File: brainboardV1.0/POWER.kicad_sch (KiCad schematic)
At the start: 16 parts, among them J21 Conn_01x01, J22 Conn_01x01, J23 Conn_01x01, U21 LD1117S18TR_SOT223

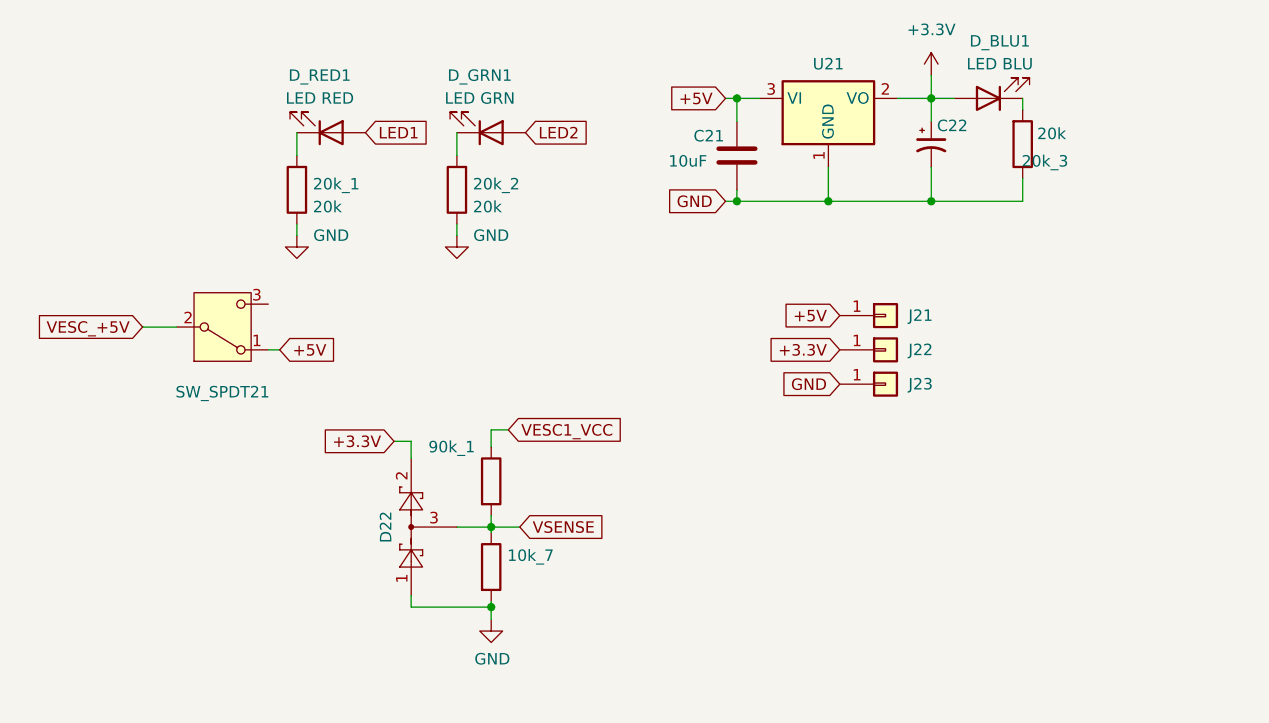
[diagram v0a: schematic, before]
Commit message: finalized PCB, changed file names
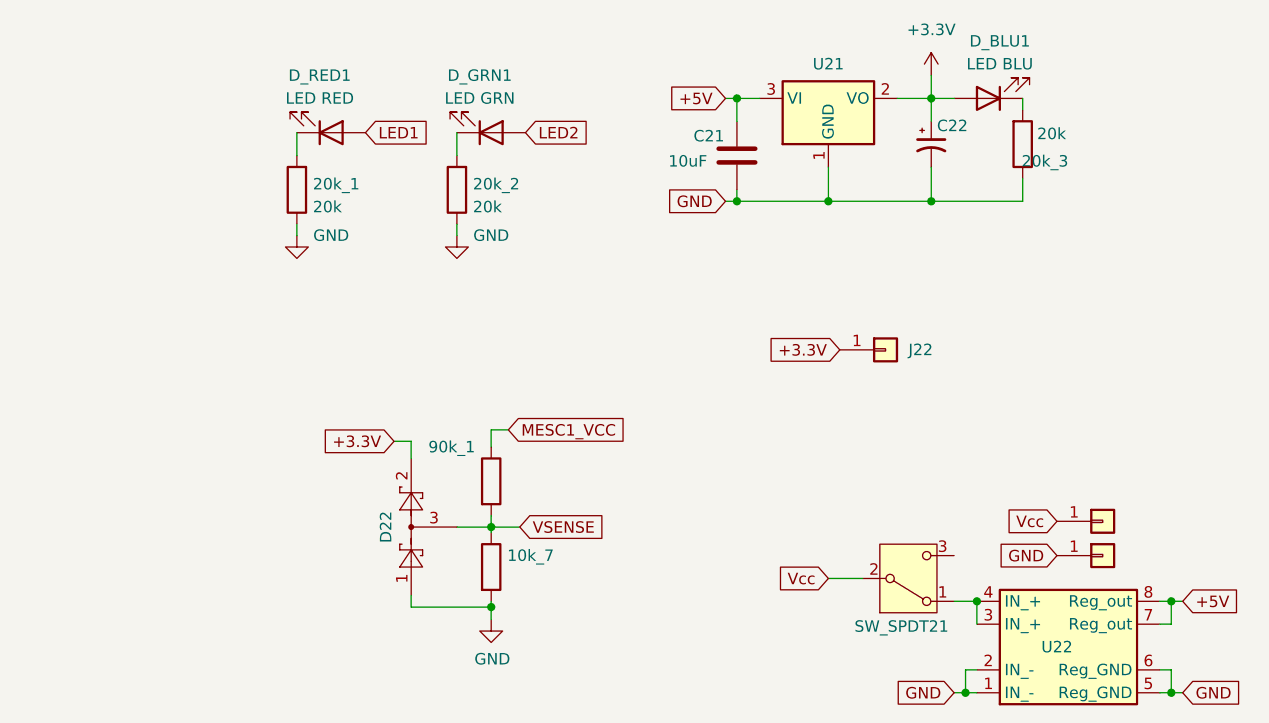
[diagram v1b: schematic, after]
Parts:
- removed J21, J23: Conn_01x01, Connector_PinSocket_2.54mm:PinSocket_1x01_P2.54mm_Vertical, symbol Connector_Generic:Conn_01x01
- added J24, J25: Conn_01x01, Connector_Wire:SolderWire-2sqmm_1x01_D2mm_OD3.9mm, symbol Connector_Generic:Conn_01x01
- added U22: my_buck_boost, Converter_DCDC:my_buck_boost, symbol two_motor_driver-rescue:my_buck_boost-Regulator_Switching
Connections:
- net +5V: now also U22.7 (Reg_out), U22.8 (Reg_out); no longer SW_SPDT21.1 (A)
- net GND: now also J24.1 (Pin_1), U22.1 (IN_-), U22.2 (IN_-), U22.5 (Reg_GND), U22.6 (Reg_GND)
- net VESC1_VCC renamed MESC1_VCC
- net VESC_+5V renamed Vcc
- net Vcc: now also J25.1 (Pin_1)
- new net: SW_SPDT21.1 (A), U22.3 (IN_+), U22.4 (IN_+)
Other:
- moved on the sheet: SW_SPDT21
